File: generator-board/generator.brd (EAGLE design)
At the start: 50 x 22.5 mm, 46 parts, among them IC1 MAX1771, Q1 IRF740DPACK

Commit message: adding part ordering numbers
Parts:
- C10, C11, C12, C13, C14, C15, C16, C4, C5, C6, C7, C8, C9: value (none) -> 100n
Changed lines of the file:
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@@
 <?xml version="1.0" encoding="utf-8"?>
 <!DOCTYPE eagle SYSTEM "eagle.dtd">
-<eagle version="6.6.0">
+<eagle version="6.5.0">
 <drawing>
 <settings>
@@
 <element name="C1" library="passives-7351" package="C0603-N" value="100n" x="12.49" y="4.19" smashed="yes" rot="R180">
 <attribute name="NAME" x="14.209078125" y="5.04890625" size="0.8128" layer="25" font="vector" ratio="14" rot="R270"/>
+<attribute name="FARNELL" value="2495332" x="12.49" y="4.19" size="1.778" layer="27" rot="R180" display="off"/>
 </element>
 <element name="J1" library="dtb" package="JST-2-TH" value="" x="3.19" y="11.81" smashed="yes" rot="R90"/>
@@
 <element name="C3" library="passives-7351" package="C0603-N" value="2.2u" x="9.325" y="4.185" smashed="yes">
 <attribute name="NAME" x="6.51609375" y="4.584078125" size="0.8128" layer="25" font="vector" ratio="14"/>
+<attribute name="FARNELL" value="2496923" x="9.325" y="4.185" size="1.778" layer="27" display="off"/>
 </element>
 <element name="D1" library="diode" package="DO35-7" value="1N4148DO35-7" x="20.25" y="10.5" smashed="yes" rot="R95">
@@
 <attribute name="FARNELL" value="1625213" x="43" y="10.5" size="1.778" layer="27" rot="R95" display="off"/>
 </element>
-<element name="C4" library="passives-7351" package="C1206-N" value="" x="21.25" y="17.5" smashed="yes">
+<element name="C4" library="passives-7351" package="C1206-N" value="100n" x="21.25" y="17.5" smashed="yes">
 <attribute name="FARNELL" value="1855877" x="21.25" y="17.5" size="1.778" layer="27" display="off"/>
 </element>
-<element name="C5" library="passives-7351" package="C1206-N" value="" x="26" y="17.5" smashed="yes">
+<element name="C5" library="passives-7351" package="C1206-N" value="100n" x="26" y="17.5" smashed="yes">
 <attribute name="FARNELL" value="1855877" x="26" y="17.5" size="1.778" layer="27" display="off"/>
 </element>
-<element name="C6" library="passives-7351" package="C1206-N" value="" x="30.75" y="17.5" smashed="yes">
+<element name="C6" library="passives-7351" package="C1206-N" value="100n" x="30.75" y="17.5" smashed="yes">
 <attribute name="FARNELL" value="1855877" x="30.75" y="17.5" size="1.778" layer="27" display="off"/>
 </element>
-<element name="C7" library="passives-7351" package="C1206-N" value="" x="35.5" y="17.5" smashed="yes">
+<element name="C7" library="passives-7351" package="C1206-N" value="100n" x="35.5" y="17.5" smashed="yes">
 <attribute name="FARNELL" value="1855877" x="35.5" y="17.5" size="1.778" layer="27" display="off"/>
 </element>
-<element name="C8" library="passives-7351" package="C1206-N" value="" x="40.25" y="17.5" smashed="yes">
+<element name="C8" library="passives-7351" package="C1206-N" value="100n" x="40.25" y="17.5" smashed="yes">
 <attribute name="FARNELL" value="1855877" x="40.25" y="17.5" size="1.778" layer="27" display="off"/>
 </element>
-<element name="C9" library="passives-7351" package="C1206-N" value="" x="42.25" y="4" smashed="yes">
+<element name="C9" library="passives-7351" package="C1206-N" value="100n" x="42.25" y="4" smashed="yes">
 <attribute name="FARNELL" value="1855877" x="42.25" y="4" size="1.778" layer="27" display="off"/>
 </element>
-<element name="C10" library="passives-7351" package="C1206-N" value="" x="37.5" y="4" smashed="yes">
+<element name="C10" library="passives-7351" package="C1206-N" value="100n" x="37.5" y="4" smashed="yes">
 <attribute name="FARNELL" value="1855877" x="37.5" y="4" size="1.778" layer="27" display="off"/>
 </element>
-<element name="C11" library="passives-7351" package="C1206-N" value="" x="32.75" y="4" smashed="yes">
+<element name="C11" library="passives-7351" package="C1206-N" value="100n" x="32.75" y="4" smashed="yes">
 <attribute name="FARNELL" value="1855877" x="32.75" y="4" size="1.778" layer="27" display="off"/>
 </element>
-<element name="C12" library="passives-7351" package="C1206-N" value="" x="28" y="4" smashed="yes">
+<element name="C12" library="passives-7351" package="C1206-N" value="100n" x="28" y="4" smashed="yes">
 <attribute name="FARNELL" value="1855877" x="28" y="4" size="1.778" layer="27" display="off"/>
 </element>
-<element name="C13" library="passives-7351" package="C1206-N" value="" x="23.25" y="4" smashed="yes">
+<element name="C13" library="passives-7351" package="C1206-N" value="100n" x="23.25" y="4" smashed="yes">
 <attribute name="FARNELL" value="1855877" x="23.25" y="4" size="1.778" layer="27" display="off"/>
 </element>
-<element name="C14" library="passives-7351" package="C1206-N" value="" x="17.5" y="5.5" smashed="yes">
+<element name="C14" library="passives-7351" package="C1206-N" value="100n" x="17.5" y="5.5" smashed="yes">
 <attribute name="FARNELL" value="1855877" x="17.5" y="5.5" size="1.778" layer="27" display="off"/>
 </element>
@@
 <attribute name="FARNELL" value="1625213" x="45.25" y="10.5" size="1.778" layer="27" rot="R265" display="off"/>
 </element>
-<element name="C15" library="passives-7351" package="C1206-N" value="" x="45" y="17.5" smashed="yes">
+<element name="C15" library="passives-7351" package="C1206-N" value="100n" x="45" y="17.5" smashed="yes">
 <attribute name="FARNELL" value="1855877" x="45" y="17.5" size="1.778" layer="27" display="off"/>
 </element>
-<element name="C16" library="passives-7351" package="C1206-N" value="" x="47" y="4" smashed="yes">
+<element name="C16" library="passives-7351" package="C1206-N" value="100n" x="47" y="4" smashed="yes">
 <attribute name="FARNELL" value="1855877" x="47" y="4" size="1.778" layer="27" display="off"/>
 </element>
@@
 <attribute name="NAME" x="4.22" y="0.595" size="0.8128" layer="25" font="vector" ratio="14" rot="R90"/>
 <attribute name="VALUE" x="2.825" y="4.28" size="1.27" layer="27" rot="R270"/>
+<attribute name="FARNELL" value="1771727" x="6" y="2.375" size="1.778" layer="27" rot="R180" display="off"/>
 </element>
 <element name="TP1" library="Testpoint" package="TP" value="TP" x="49" y="1.5"/>

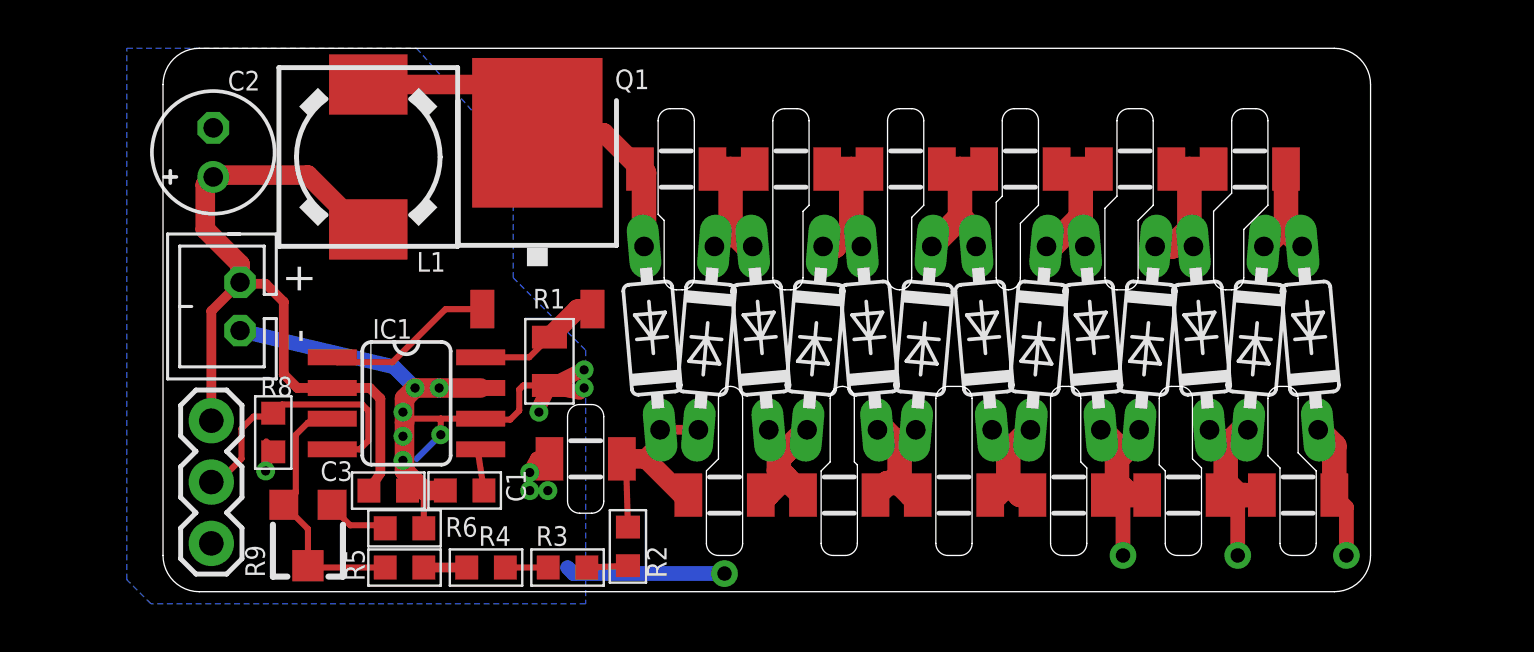
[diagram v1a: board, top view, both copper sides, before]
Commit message: almost done
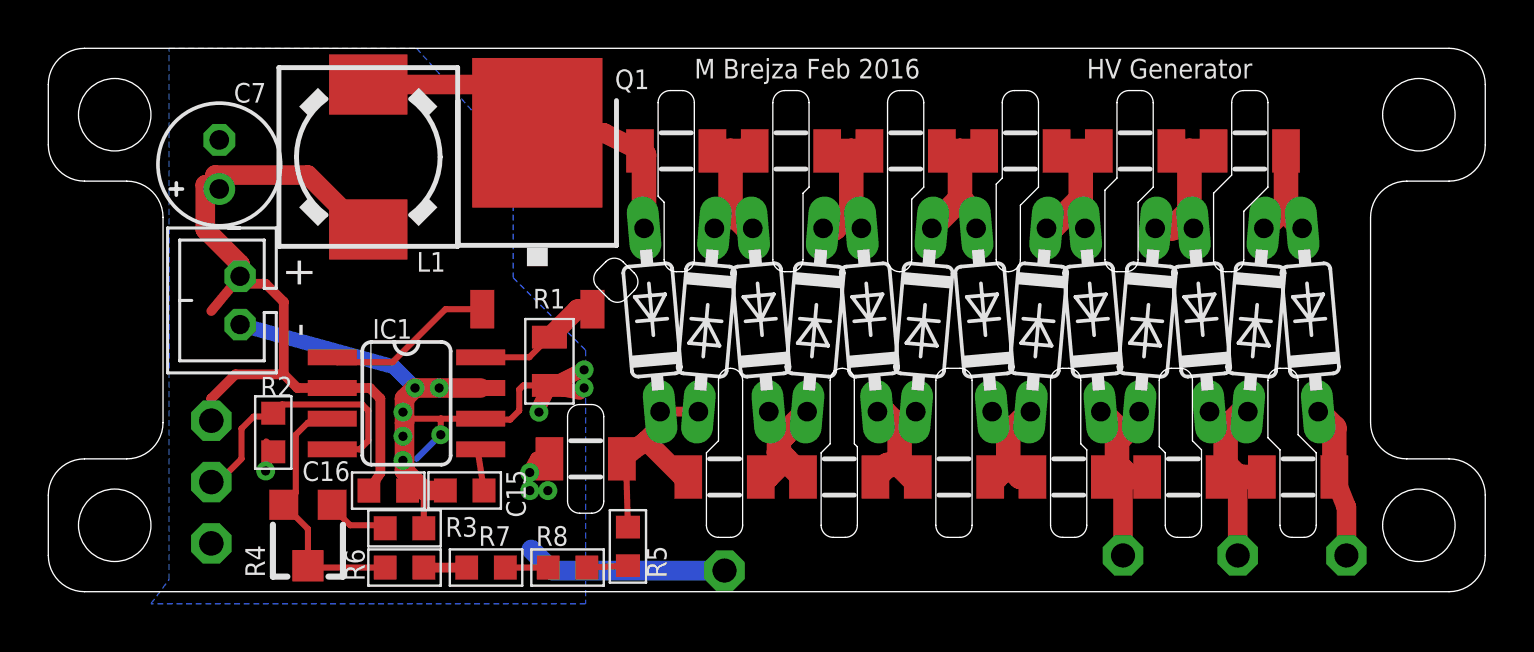
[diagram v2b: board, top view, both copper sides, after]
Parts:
- removed JP1: (no value), SparkFun-Connectors:1X03
- removed R9: 47k, rcl:RTRIM3103
- removed TP1, TP2, TP3, TP4: TP, Testpoint:TP
- added J2: HV_GEN-HOLE, generator-lib:BRD-LAYOUT2
- added R7: 6.8M, passives-7351:R0603-N
- C1: device passives-7351:C0603-N -> passives-7351:C1206-N
- C15: device passives-7351:C1206-N -> passives-7351:C0603-N
- C16: value 100n -> 2.2u; device passives-7351:C1206-N -> passives-7351:C0603-N
- C2: value 47u -> 100n; device rcl:E2-5 -> passives-7351:C1206-N
- C3: value 2.2u -> 100n; device passives-7351:C0603-N -> passives-7351:C1206-N
- C7: value 100n -> 47u; device passives-7351:C1206-N -> rcl:E2-5
- R2: value 6.8M -> 100k
- R3: value 6.8M -> 560k
- R4: value 6.8M -> 47k; device passives-7351:R0603-N -> rcl:RTRIM3103
- R6: value 560k -> 6.8M
- R8: value 100k -> 6.8M
- moved C16 37.7 mm to (9.32, 4.18)
- moved C15 35.1 mm to (12.5, 4.19), turned to 180 degrees
- moved C7 33.2 mm to (2.33, 17.7), turned to 90 degrees
- moved C14 29.5 mm to (47.0, 4.75)
- moved C8 25.7 mm to (17.5, 5.50)
- moved C3 25.6 mm to (30.8, 18.2)
- moved C2 23.9 mm to (26.0, 18.2), turned to 0 degrees
- moved C13 19.0 mm to (42.2, 4.75)
- moved C9 19.0 mm to (23.2, 4.75)
- moved C1 16.6 mm to (21.2, 18.2), turned to 0 degrees
- moved R2 15.4 mm to (4.57, 6.59)
- moved C4 14.3 mm to (35.5, 18.2)
- moved C5 14.3 mm to (40.2, 18.2)
- moved C6 14.3 mm to (45.0, 18.2)
- moved R8 13.4 mm to (16.8, 1.00), turned to 0 degrees
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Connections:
- removed net N$24: IC1.4, JP1.2, R8.2
- removed net N$4: C2.+, C3.1, IC1.2, J1.1, JP1.3, L1.2
- new net SHDN: IC1.4, J2.SHDN, R2.2
- new net VIN: C16.1, C7.+, IC1.2, J1.1, J2.VIN, L1.2
- net GND: now also C15.2, C16.2, C7.-, C8.1, J2.GND_HV, J2.GND_LV, R2.1, R3.2; no longer C1.2, C14.1, C2.-, C3.2, JP1.1, R6.2, R8.1, TP4.P$1
- net N$10: now also C10.2; no longer C12.2
- net N$11: now also C3.2, C4.1; no longer C6.2, C7.1
- net N$12: now also C12.1; no longer C10.1
- net N$13: now also C4.2, C5.1; no longer C7.2, C8.1
- net N$14: now also C12.2, C13.1, J2.HV1; no longer C10.2, C9.1, TP3.P$1
- net N$15: now also C5.2, C6.1; no longer C15.1, C8.2
- net N$16: now also C13.2, C14.1, J2.HV2; no longer C16.1, C9.2, TP2.P$1
- net N$17: now also R4.2, R4.3, R6.1; no longer R5.1, R9.2, R9.3
- net N$18: now also R5.1, R8.2; no longer R2.1, R3.2
- net N$19: now also R7.2, R8.1; no longer R3.1, R4.2
- net N$20: now also R6.2, R7.1; no longer R4.1, R5.2
- net N$23: now also R3.1, R4.1; no longer R6.1, R9.1
- net N$25: now also C6.2; no longer C15.2
- net N$26: now also C14.2, J2.HV3; no longer C16.2, TP1.P$1
- net N$3: now also C8.2, C9.1, R5.2; no longer C13.1, C14.2, R2.2
- net N$5: now also C15.1; no longer C1.1
- net N$6: now also C1.1; no longer C4.1
- net N$7: now also C1.2, C2.1; no longer C4.2, C5.1
- net N$8: now also C10.1, C9.2; no longer C12.1, C13.2
- net N$9: now also C2.2, C3.1; no longer C5.2, C6.1
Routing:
- net VIN: track 0.00 -> 32.8 mm
- net N$4: track 32.2 -> 0.00 mm
- net SHDN: track 0.00 -> 11.6 mm
- net N$24: track 11.6 -> 0.00 mm
- net GND: track 37.5 -> 39.3 mm
- net N$16: track 8.61 -> 9.36 mm
- net N$26: track 5.69 -> 6.33 mm
- net N$14: track 9.13 -> 9.73 mm
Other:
- board size 50 x 22.5 mm -> 59.5 x 22.5 mm
- board text added: "GND"
- board text added: "HV Generator"
- board text added: "M Brejza Feb 2016"
- board text added: "SHDN"
- board text added: "Vin"
